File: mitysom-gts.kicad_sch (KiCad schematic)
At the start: 29 parts, among them J1 Plug_Samtec_SEAM-50-02.0-L-08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

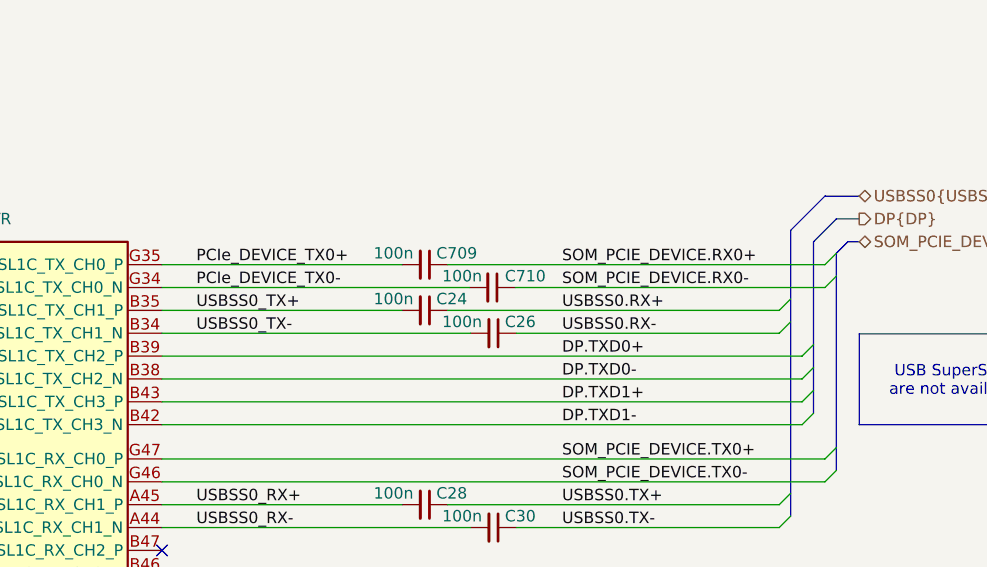
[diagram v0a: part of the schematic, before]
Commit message: [#101340] Add flash sockets
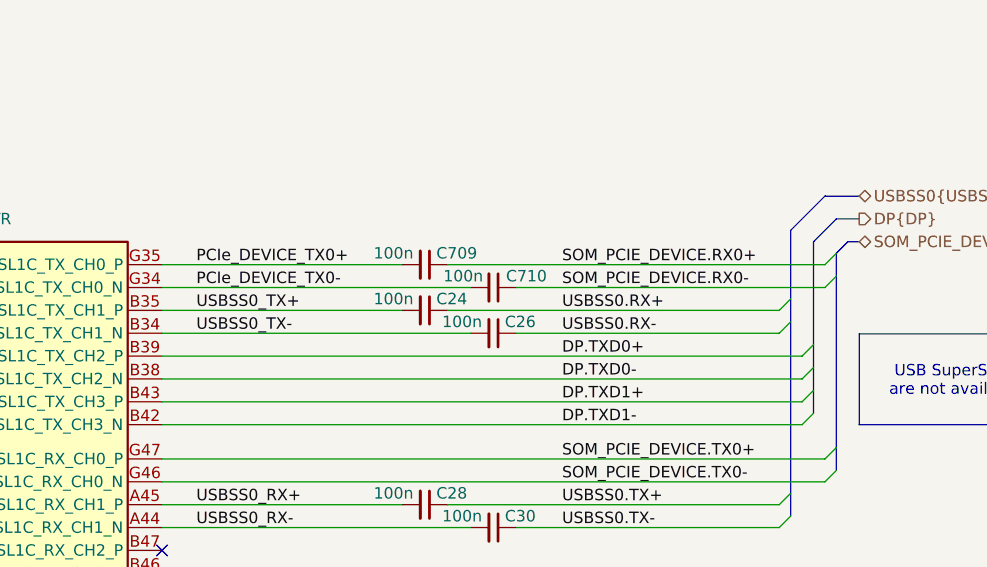
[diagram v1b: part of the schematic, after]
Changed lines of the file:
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@@
 	(wire
 		(pts
-			(xy 281.8161 109.22) (xy 316.23 109.22)
+			(xy 281.94 109.22) (xy 316.23 109.22)
 		)
 		(stroke
@@
 	(wire
 		(pts
-			(xy 242.57 109.22) (xy 276.7361 109.22)
+			(xy 242.57 109.22) (xy 276.86 109.22)
 		)
 		(stroke
@@
 	(symbol
 		(lib_id "antmicroCapacitors0402:C_100n_0402")
-		(at 281.8161 109.22 0)
+		(at 281.94 109.22 0)
 		(mirror y)
 		(unit 1)
@@
 		(dnp no)
 		(property "Reference" "C710"
-			(at 280.67 107.95 0)
+			(at 280.7939 107.95 0)
 			(show_name no)
 			(do_not_autoplace no)
@@
 		)
 		(property "Value" "C_100n_0402"
-			(at 261.4961 119.38 0)
+			(at 261.62 119.38 0)
 			(hide yes)
 			(show_name no)
@@
 		)
 		(property "Footprint" "antmicro-footprints:C_0402_1005Metric"
-			(at 261.4961 121.92 0)
+			(at 261.62 121.92 0)
 			(hide yes)
 			(show_name no)
@@
 		)
 		(property "Datasheet" "https://www.murata.com/products/productdetail?partno=GRM155R61H104KE14%23"
-			(at 261.4961 124.46 0)
+			(at 261.62 124.46 0)
 			(hide yes)
 			(show_name no)
@@
 		)
 		(property "Description" "SMD Multilayer Ceramic Capacitor, 0.1 µF, 50 V, 0402 [1005 Metric], ± 10%, X5R, GRM Series"
-			(at 281.8161 109.22 0)
+			(at 281.94 109.22 0)
 			(hide yes)
 			(show_name no)
@@
 		)
 		(property "MPN" "GRM155R61H104KE14D"
-			(at 261.4961 127 0)
+			(at 261.62 127 0)
 			(hide yes)
 			(show_name no)
@@
 		)
 		(property "Manufacturer" "Murata"
-			(at 261.4961 129.54 0)
+			(at 261.62 129.54 0)
 			(hide yes)
 			(show_name no)
@@
 		)
 		(property "License" "Apache-2.0"
-			(at 261.4961 132.08 0)
+			(at 261.62 132.08 0)
 			(hide yes)
 			(show_name no)
@@
 		)
 		(property "Author" "Antmicro"
-			(at 261.4961 134.62 0)
+			(at 261.62 134.62 0)
 			(hide yes)
 			(show_name no)
@@
 		)
 		(property "Val" "100n"
-			(at 278.13 107.95 0)
+			(at 278.2539 107.95 0)
 			(show_name no)
 			(do_not_autoplace no)
@@
 		)
 		(property "Voltage" "50V"
-			(at 261.4961 137.16 0)
+			(at 261.62 137.16 0)
 			(hide yes)
 			(show_name no)
@@
 		)
 		(property "Dielectric" "X5R"
-			(at 261.4961 139.7 0)
+			(at 261.62 139.7 0)
 			(hide yes)
 			(show_name no)
